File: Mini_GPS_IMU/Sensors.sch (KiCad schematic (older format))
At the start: 7 parts, among them U3 SAM-M8Q, U4 MPU-9250, U5 MS5611

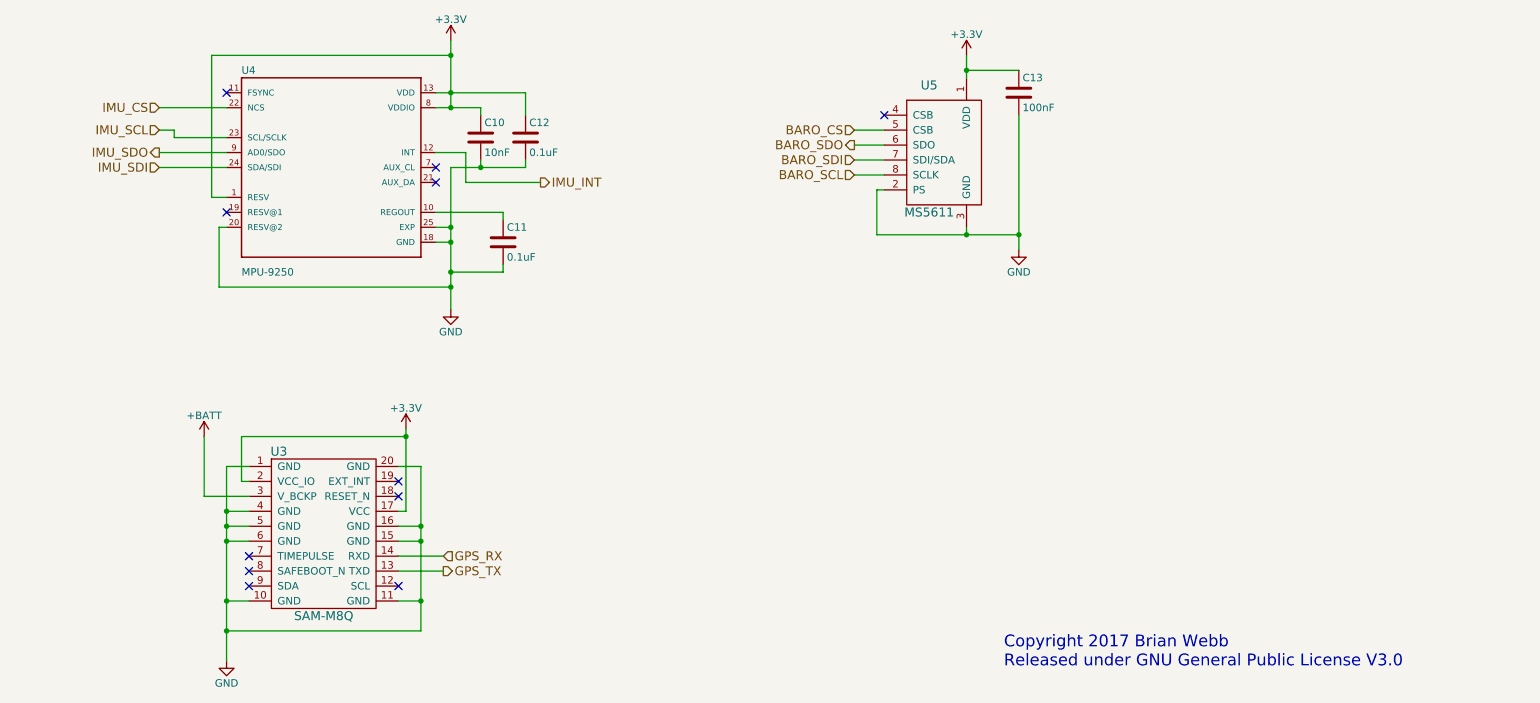
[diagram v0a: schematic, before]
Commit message: Finished version 1.0 of GPS Diamond.
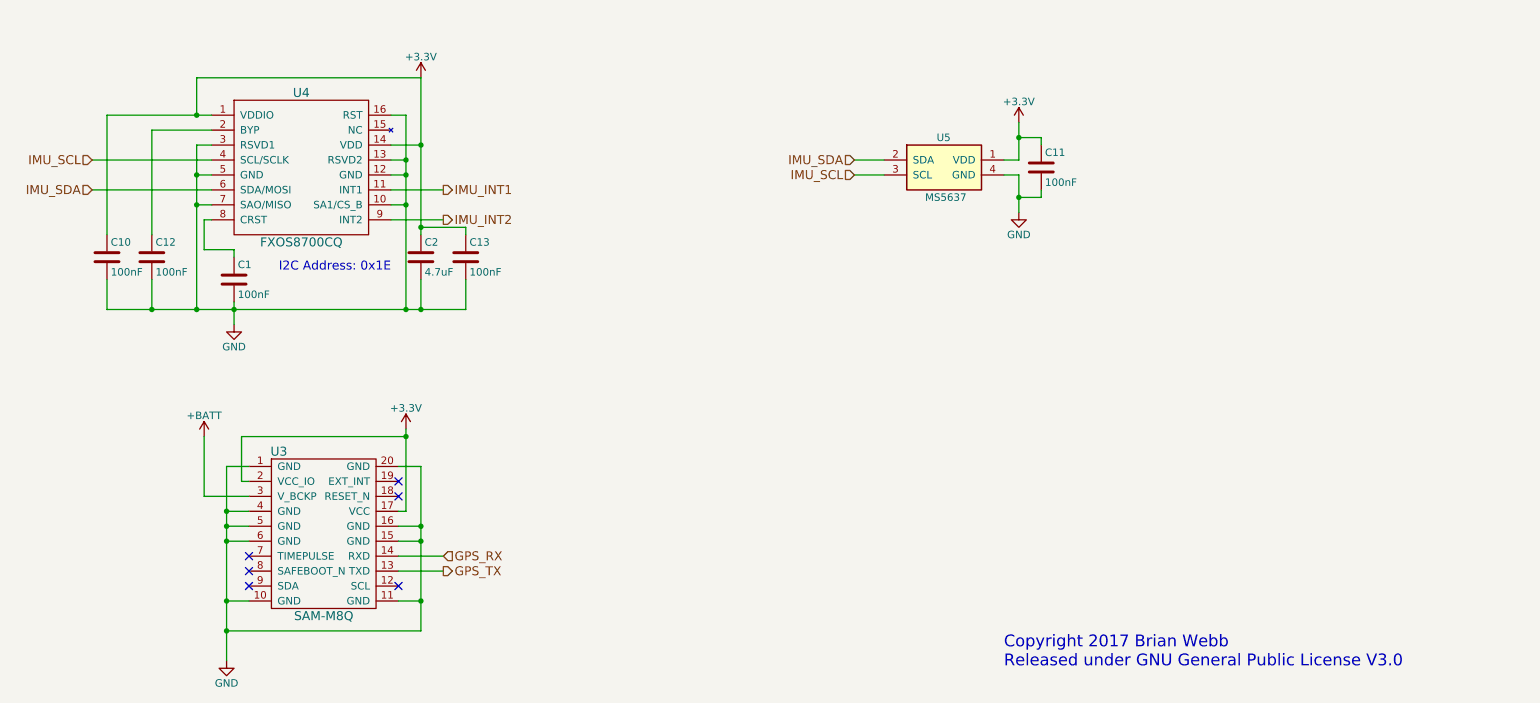
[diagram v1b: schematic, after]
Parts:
- removed U4: MPU-9250, MPU-9250:QFN40P300X300X105-25N, symbol MPU-9250
- removed U5: MS5611, local:MS5611, symbol MS5611
- added C1: 100nF, Capacitors_SMD:C_0402, symbol C
- added C2: 4.7uF, Capacitors_SMD:C_0402, symbol C
- added U4: FXOS8700CQ, local:FXOS8700CQ, symbol FXOS8700CQ
- added U5: MS5637, local:MS5637, symbol MS5637
- C10: value 10nF -> 100nF; footprint Capacitors_SMD:C_0402_NoSilk -> Capacitors_SMD:C_0402
- C11: value 0.1uF -> 100nF
- C12: value 0.1uF -> 100nF; footprint Capacitors_SMD:C_0402_NoSilk -> Capacitors_SMD:C_0402
- C13: footprint Capacitors_SMD:C_0402_NoSilk -> Capacitors_SMD:C_0402
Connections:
- net +3V3: now also C11.1, C2.1, U4.1 (VDDIO), U4.14 (VDD), U5.1 (VDD); no longer C12.1
- net GND: now also C1.2, C2.2, U4.10 (SA1/CS_B), U4.12 (GND), U4.13 (RSVD2), U4.16 (RST), U4.3 (RSVD1), U4.5 (GND), U4.7 (SAO/MISO), U5.4 (GND)
- net IMU_SCL: now also U4.4 (SCL/SCLK), U5.3 (SCL)
- new net: C12.1, U4.2 (BYP)
- new net: C1.1, U4.8 (CRST)
- new net IMU_INT1: U4.11 (INT1)
- new net IMU_INT2: U4.9 (INT2)
- new net IMU_SDA: U4.6 (SDA/MOSI), U5.2 (SDA)
- no-connect marks 11 -> 6
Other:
- note added: "I2C Address: 0x1E"
- moved on the sheet: C10, C11, C12
